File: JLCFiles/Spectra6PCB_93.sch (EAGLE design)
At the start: 97 parts, among them J5 NC, P1 FH12-50S-0.5SH, Q1 310mA/60V/1.6Ω, Q2 20V/4.2A/52mΩ/1.4W, Q3 DMG3415U, U1 GENERIC-SOIC8MSGEQ7N-FILTER, U2 AP2112, U3 ESP-WROOM-3232D-NARROW, U4 MP6211 3.3V

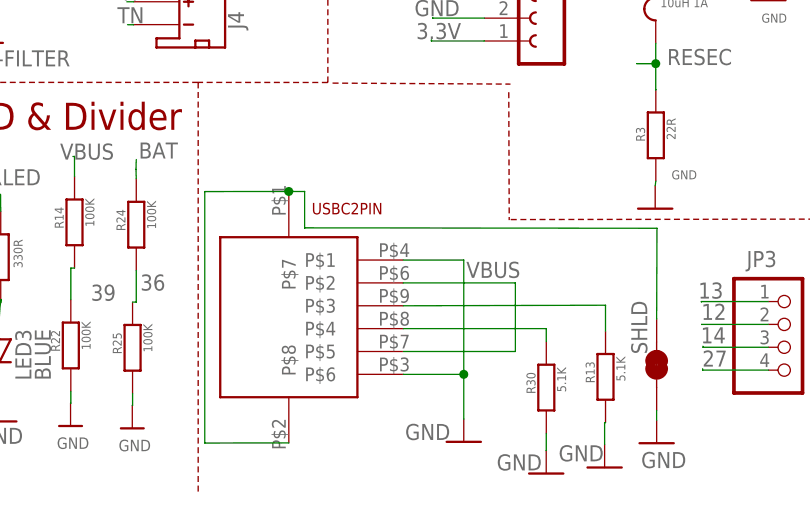
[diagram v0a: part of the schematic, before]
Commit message: JLCPCB
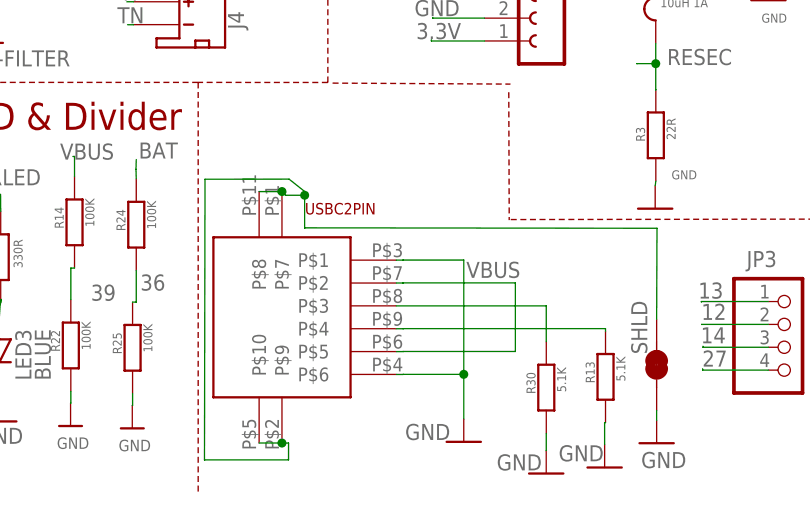
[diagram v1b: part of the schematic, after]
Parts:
- U$4: device USBC6PIN4:USBC6PIN -> USBC6PIN2:USBC6PIN
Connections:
- net N$41: now also R13.2; no longer R30.2
- net N$42: now also R30.2; no longer R13.2
- net SHLD: now also U$4.P$10, U$4.P$9
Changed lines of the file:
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@@
 <part name="U4" library="microbuilder" deviceset="VREG_SOT23-5" device="" value="MP6211 3.3V"/>
 <part name="JP4" library="SparkFun-Jumpers" deviceset="JUMPER-SMT_3_1-NC_TRACE" device="_SILK" package3d_urn="urn:adsk.eagle:package:39288/1"/>
-<part name="U$4" library="USBC6PIN4" deviceset="USBC6PIN" device=""/>
 <part name="GND13" library="SparkFun-PowerSymbols" deviceset="GND" device=""/>
 <part name="R30" library="rcl" library_urn="urn:adsk.eagle:library:334" deviceset="R-EU_" device="M0805" package3d_urn="urn:adsk.eagle:package:23556/2" value="5.1K"/>
@@
 <part name="JP7" library="SparkFun-Jumpers" deviceset="JUMPER-SMT_3_1-NC_TRACE" device="_SILK" package3d_urn="urn:adsk.eagle:package:39288/1"/>
 <part name="SV3" library="con-lsta" library_urn="urn:adsk.eagle:library:161" deviceset="FE05-1" device="" package3d_urn="urn:adsk.eagle:package:8190/1"/>
+<part name="U$4" library="USBC6PIN2" deviceset="USBC6PIN" device=""/>
 </parts>
 <sheets>
@@
 <attribute name="VALUE" x="38.394" y="59.33" size="1.778" layer="96" font="vector" align="center"/>
 </instance>
-<instance part="U$4" gate="G$1" x="115.47" y="26.35" smashed="yes"/>
 <instance part="GND13" gate="1" x="137.45" y="11.23" smashed="yes">
 <attribute name="VALUE" x="133.44" y="13.216" size="1.778" layer="96" font="vector" align="top-center"/>
@@
 <attribute name="NAME" x="227.25" y="13.108" size="1.778" layer="95" rot="R180"/>
 </instance>
+<instance part="U$4" gate="G$1" x="114.71" y="26.34" smashed="yes"/>
 </instances>
 <busses>
@@
 </segment>
 <segment>
-<pinref part="U$4" gate="G$1" pin="P$1"/>
 <wire x1="130.71" y1="31.43" x2="137.45" y2="31.43" width="0.1524" layer="91"/>
 <wire x1="137.45" y1="31.43" x2="137.45" y2="18.73" width="0.1524" layer="91"/>
-<pinref part="U$4" gate="G$1" pin="P$6"/>
 <wire x1="137.45" y1="18.73" x2="137.45" y2="13.77" width="0.1524" layer="91"/>
 <wire x1="130.71" y1="18.73" x2="137.45" y2="18.73" width="0.1524" layer="91"/>
 <junction x="137.45" y="18.73"/>
 <pinref part="GND13" gate="1" pin="GND"/>
+<pinref part="U$4" gate="G$1" pin="P$1"/>
+<wire x1="129.95" y1="31.42" x2="130.71" y2="31.42" width="0.1524" layer="91"/>
+<wire x1="130.71" y1="31.42" x2="130.71" y2="31.43" width="0.1524" layer="91"/>
+<pinref part="U$4" gate="G$1" pin="P$6"/>
+<wire x1="129.95" y1="18.72" x2="130.71" y2="18.72" width="0.1524" layer="91"/>
+<wire x1="130.71" y1="18.72" x2="130.71" y2="18.73" width="0.1524" layer="91"/>
 </segment>
 <segment>
@@
 </segment>
 <segment>
-<pinref part="U$4" gate="G$1" pin="P$5"/>
 <wire x1="130.71" y1="21.27" x2="143.18" y2="21.27" width="0.1524" layer="91"/>
 <wire x1="143.18" y1="21.27" x2="143.18" y2="28.89" width="0.1524" layer="91"/>
-<pinref part="U$4" gate="G$1" pin="P$2"/>
 <wire x1="143.18" y1="28.89" x2="130.71" y2="28.89" width="0.1524" layer="91"/>
 <label x="137.73" y="29.45" size="1.778" layer="95"/>
+<pinref part="U$4" gate="G$1" pin="P$2"/>
+<wire x1="129.95" y1="28.88" x2="130.71" y2="28.88" width="0.1524" layer="91"/>
+<wire x1="130.71" y1="28.88" x2="130.71" y2="28.89" width="0.1524" layer="91"/>
+<pinref part="U$4" gate="G$1" pin="P$5"/>
+<wire x1="129.95" y1="21.26" x2="130.71" y2="21.26" width="0.1524" layer="91"/>
+<wire x1="130.71" y1="21.26" x2="130.71" y2="21.27" width="0.1524" layer="91"/>
 </segment>
 <segment>
@@
 <net name="SHLD" class="0">
 <segment>
-<pinref part="U$4" gate="G$1" pin="P$7"/>
-<pinref part="U$4" gate="G$1" pin="P$8"/>
-<wire x1="118.01" y1="11.11" x2="108.67" y2="11.1" width="0.1524" layer="91"/>
-<wire x1="108.67" y1="11.1" x2="108.67" y2="39.04" width="0.1524" layer="91"/>
-<wire x1="108.67" y1="39.04" x2="118.01" y2="39.05" width="0.1524" layer="91"/>
-<wire x1="118.01" y1="39.05" x2="119.77" y2="39.05" width="0.1524" layer="91"/>
-<junction x="118.01" y="39.05"/>
-<wire x1="119.77" y1="39.05" x2="119.77" y2="35.01" width="0.1524" layer="91"/>
+<wire x1="117.98" y1="9.23" x2="108.64" y2="9.22" width="0.1524" layer="91"/>
+<wire x1="108.64" y1="9.22" x2="108.7" y2="40.41" width="0.1524" layer="91"/>
+<wire x1="108.7" y1="40.41" x2="118.04" y2="40.42" width="0.1524" layer="91"/>
+<wire x1="118.04" y1="40.42" x2="119.77" y2="39.05" width="0.1524" layer="91"/>
+<wire x1="119.77" y1="39.05" x2="119.77" y2="38.63" width="0.1524" layer="91"/>
+<wire x1="119.77" y1="38.63" x2="119.77" y2="35.01" width="0.1524" layer="91"/>
 <wire x1="119.77" y1="35.01" x2="119.81" y2="35.01" width="0.1524" layer="91"/>
 <pinref part="SHLD" gate="G$1" pin="2"/>
 <wire x1="119.77" y1="35.01" x2="158.92" y2="34.96" width="0.1524" layer="91"/>
 <wire x1="158.92" y1="34.96" x2="158.88" y2="24.87" width="0.1524" layer="91"/>
+<pinref part="U$4" gate="G$1" pin="P$10"/>
+<pinref part="U$4" gate="G$1" pin="P$9"/>
+<wire x1="114.71" y1="11.1" x2="117.25" y2="11.1" width="0.1524" layer="91"/>
+<wire x1="117.25" y1="11.1" x2="117.98" y2="11.1" width="0.1524" layer="91"/>
+<wire x1="117.98" y1="11.1" x2="117.98" y2="9.23" width="0.1524" layer="91"/>
+<junction x="117.25" y="11.1"/>
+<pinref part="U$4" gate="G$1" pin="P$8"/>
+<pinref part="U$4" gate="G$1" pin="P$7"/>
+<wire x1="114.71" y1="39.04" x2="117.25" y2="39.04" width="0.1524" layer="91"/>
+<wire x1="117.25" y1="39.04" x2="117.66" y2="38.63" width="0.1524" layer="91"/>
+<wire x1="117.66" y1="38.63" x2="119.77" y2="38.63" width="0.1524" layer="91"/>
+<junction x="117.25" y="39.04"/>
+<junction x="119.77" y="38.63"/>
 </segment>
 </net>
@@
 </segment>
 </net>
-<net name="N$42" class="0">
-<segment>
-<pinref part="U$4" gate="G$1" pin="P$3"/>
+<net name="N$41" class="0">
+<segment>
+<wire x1="130.71" y1="23.81" x2="146.6" y2="23.81" width="0.1524" layer="91"/>
+<pinref part="U$4" gate="G$1" pin="P$4"/>
+<wire x1="146.6" y1="23.81" x2="146.62" y2="23.81" width="0.1524" layer="91"/>
+<wire x1="129.95" y1="23.8" x2="130.71" y2="23.8" width="0.1524" layer="91"/>
+<wire x1="130.71" y1="23.8" x2="130.71" y2="23.81" width="0.1524" layer="91"/>
 <pinref part="R13" gate="G$1" pin="2"/>
-<wire x1="130.71" y1="26.35" x2="153.2" y2="26.41" width="0.1524" layer="91"/>
-<wire x1="153.2" y1="26.41" x2="153.2" y2="23.53" width="0.1524" layer="91"/>
-</segment>
-</net>
-<net name="N$41" class="0">
-<segment>
-<pinref part="U$4" gate="G$1" pin="P$4"/>
-<pinref part="R30" gate="G$1" pin="2"/>
-<wire x1="130.71" y1="23.81" x2="146.62" y2="23.81" width="0.1524" layer="91"/>
-<wire x1="146.62" y1="23.81" x2="146.62" y2="22.34" width="0.1524" layer="91"/>
+<wire x1="153.2" y1="23.53" x2="153.2" y2="23.81" width="0.1524" layer="91"/>
+<wire x1="153.2" y1="23.81" x2="146.62" y2="23.81" width="0.1524" layer="91"/>
 </segment>
 </net>
@@
 </segment>
 </net>
+<net name="N$42" class="0">
+<segment>
+<pinref part="U$4" gate="G$1" pin="P$3"/>
+<pinref part="R30" gate="G$1" pin="2"/>
+<wire x1="129.95" y1="26.34" x2="146.62" y2="26.34" width="0.1524" layer="91"/>
+<wire x1="146.62" y1="26.34" x2="146.62" y2="22.34" width="0.1524" layer="91"/>
+</segment>
+</net>
